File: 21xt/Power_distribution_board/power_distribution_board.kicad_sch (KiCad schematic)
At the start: 38 parts, among them IC1 LM74700QDBVRQ1, IC2 LM74700QDBVRQ1, IC3 LTC2959IDDB#TRMPBF, IC4 INA180A1IDBVR, IC5 TLV76150DCYR, J1 Conn_01x02, J2 Conn_01x02, J3 Conn_01x02, J4 Conn_01x02, J5 Conn_01x02, Q1 NVMFWS2D1N08XT1G, Q2 NVMFWS2D1N08XT1G, Q3 NVMFWS2D1N08XT1G, U1 esp32 c6 xiao, U2 LMV331

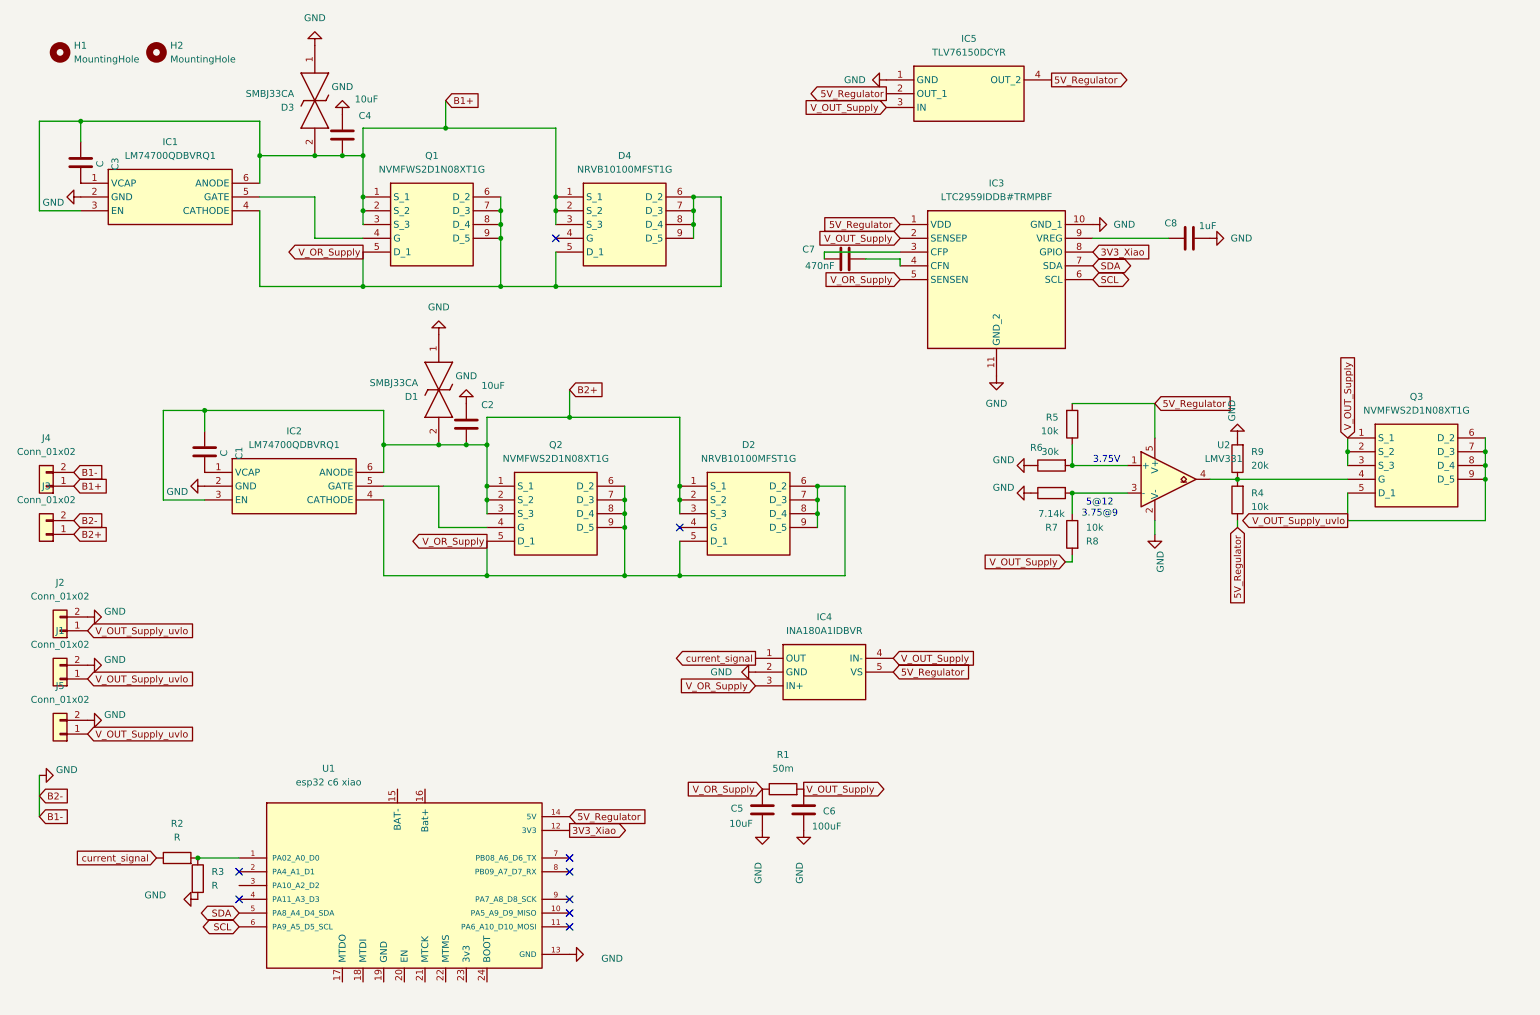
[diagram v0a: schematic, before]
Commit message: done i hope
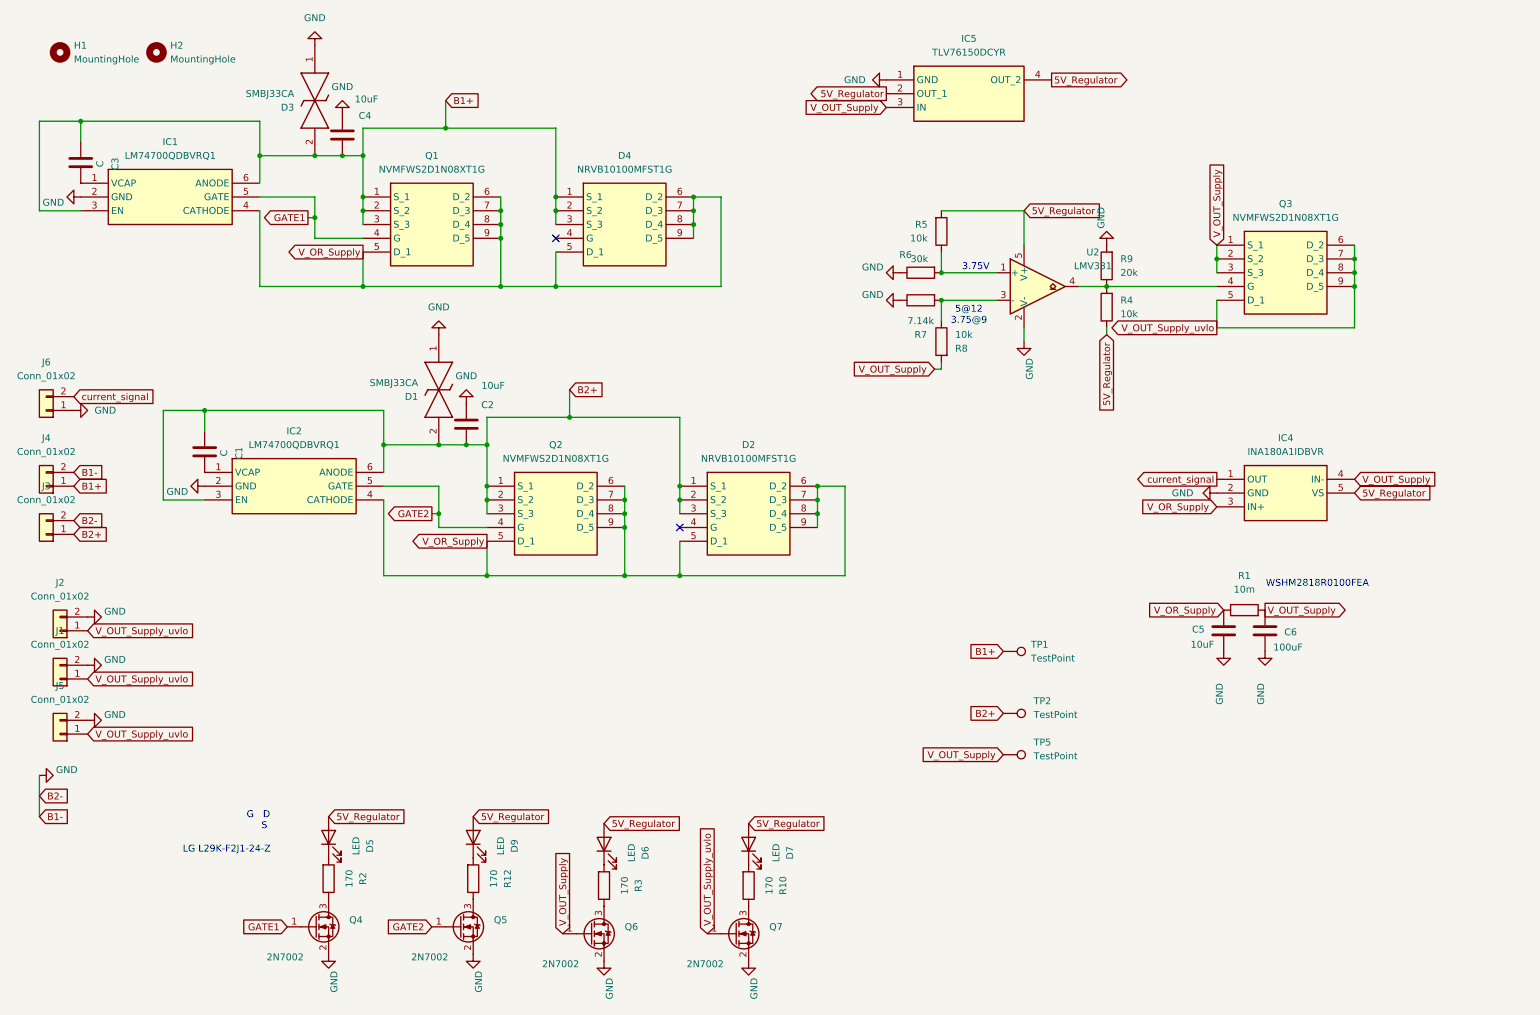
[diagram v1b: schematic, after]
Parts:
- removed C7: 470nF, Capacitor_SMD:C_0402_1005Metric, symbol Device:C
- removed C8: 1uF, Capacitor_SMD:C_0402_1005Metric, symbol Device:C
- removed IC3: LTC2959IDDB#TRMPBF, 21xt_footprints:LTC2959IDDB#TRMPBF, symbol 21xt_symbols:LTC2959IDDB#TRMPBF
- removed U1: esp32 c6 xiao, 21xt_footprints:esp32 c6 smt, symbol 21xt_symbols:102010388
- added D5, D6, D7, D9: LED, LED_SMD:LED_0603_1608Metric, symbol Device:LED
- added J6: Conn_01x02, Connector_JST:JST_EH_S2B-EH_1x02_P2.50mm_Horizontal, symbol Connector_Generic:Conn_01x02
- added Q4, Q5, Q6, Q7: 2N7002, Package_TO_SOT_SMD:SOT-23, symbol Transistor_FET:2N7002
- added R10, R12: 170, Resistor_SMD:R_0402_1005Metric, symbol Device:R
- added TP1, TP2, TP5: TestPoint, TestPoint:TestPoint_Pad_1.0x1.0mm, symbol Connector:TestPoint
- R1: value 50m -> 10m
- R2, R3: value R -> 170
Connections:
- net 5V_Regulator: now also D5.2 (A), D6.2 (A), D7.2 (A), D9.2 (A)
- net B1+: now also TP1.1
- net B2+: now also TP2.1
- net GND: now also J6.1 (Pin_1), Q4.2 (S), Q5.2 (S), Q6.2 (S), Q7.2 (S); no longer R3.2
- net V_OUT_Supply: now also Q6.1 (G), TP5.1
- net V_OUT_Supply_uvlo: now also Q7.1 (G)
- net current_signal: now also J6.2 (Pin_2); no longer R2.1
- net GATE2: now reaches IC2.5 (GATE), Q2.4 (G)
- net GATE2: now also Q5.1 (G)
- net at R3.1: now also Q6.3 (D); no longer R2.2
- net GATE1: now reaches IC1.5 (GATE), Q1.4 (G)
- net GATE1: now also Q4.1 (G)
- new net: Q7.3 (D), R10.1
- new net: D7.1 (K), R10.2
- new net: D5.1 (K), R2.2
- new net: Q5.3 (D), R12.1
- new net: D6.1 (K), R3.2
- new net: Q4.3 (D), R2.1
- new net: D9.1 (K), R12.2
- no-connect marks 9 -> 2
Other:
- note added: "G D S"
- note added: "LG L29K-F2J1-24-Z"
- note added: "WSHM2818R0100FEA"
- moved on the sheet: C5, C6, IC4, Q3, R1, R4, R5, R6, R7, R8, R9, U2

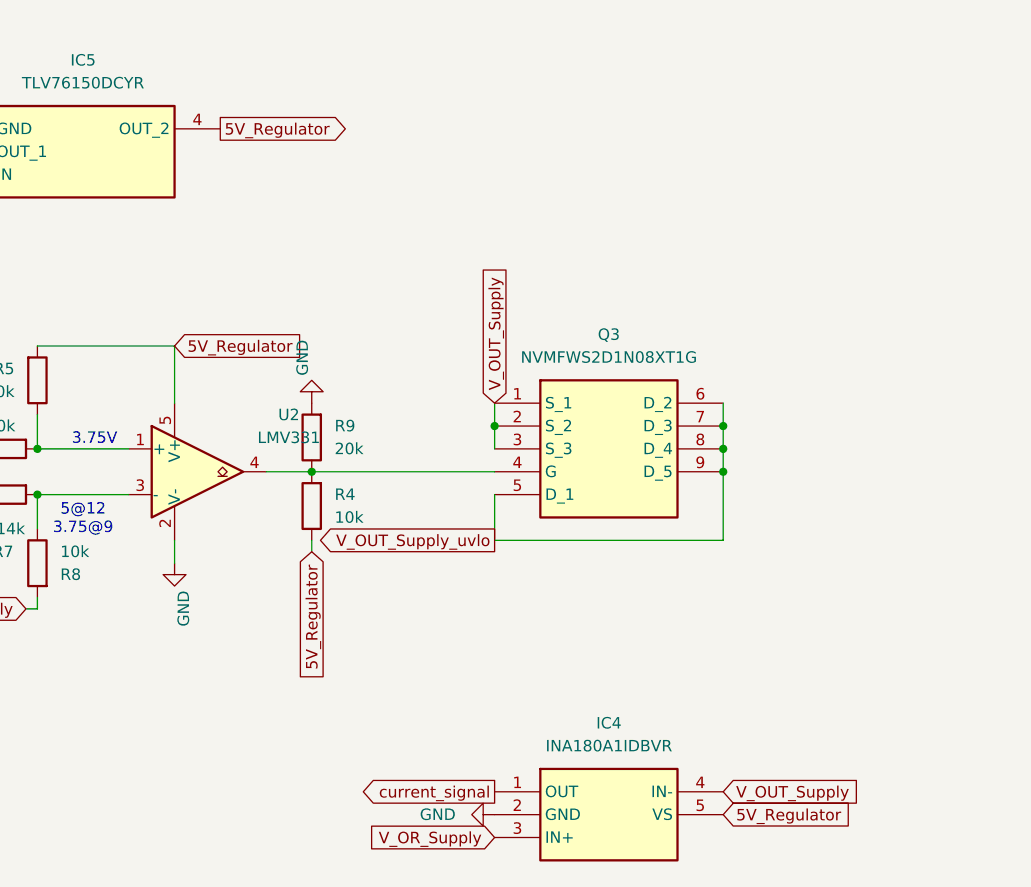
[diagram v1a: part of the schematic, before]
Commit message: adf
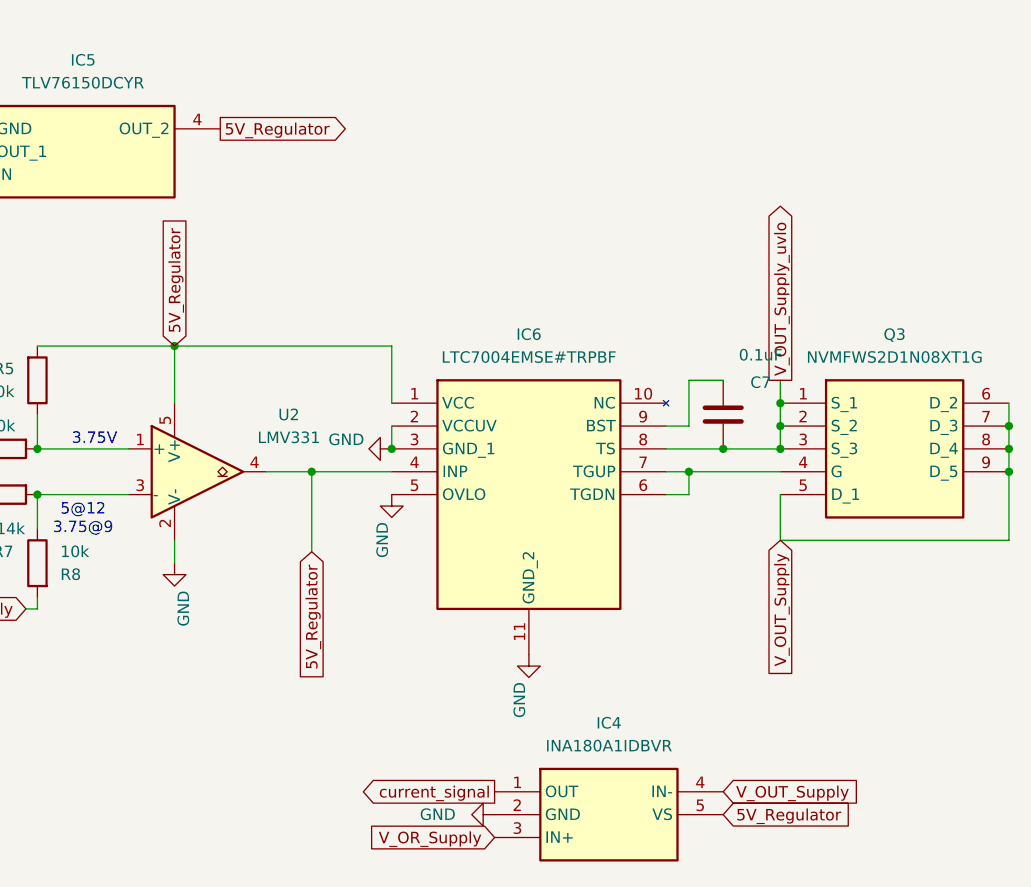
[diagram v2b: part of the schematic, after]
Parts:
- removed R4: 10k, Resistor_SMD:R_0402_1005Metric, symbol Device:R
- removed R9: 20k, Resistor_SMD:R_0402_1005Metric, symbol Device:R
- added C7: 0.1uF, Capacitor_SMD:C_0402_1005Metric, symbol Device:C
- added IC6: LTC7004EMSE#TRPBF, deans_fp:SOP50P490X110-11N, symbol ihatekicad:LTC7004EMSE#TRPBF
- J1, J2, J5: footprint 21xt_footprints:Deans Connector Female -> deans_fp:Deans Connector Female
- J3, J4: footprint 21xt_footprints:Deans Connector Male -> deans_fp:Deans Connector Male
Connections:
- net 5V_Regulator: now also U2.4, IC6.1 (VCC), IC6.4 (INP)
- net GND: now also IC6.11 (GND_2), IC6.2 (VCCUV), IC6.3 (GND_1), IC6.5 (OVLO)
- net V_OUT_Supply: now also Q3.5 (D_1), Q3.6 (D_2), Q3.7 (D_3), Q3.8 (D_4), Q3.9 (D_5); no longer Q3.1 (S_1), Q3.2 (S_2), Q3.3 (S_3)
- net V_OUT_Supply_uvlo: now also Q3.1 (S_1), Q3.2 (S_2), Q3.3 (S_3), C7.2, IC6.8 (TS); no longer Q3.5 (D_1), Q3.6 (D_2), Q3.7 (D_3), Q3.8 (D_4), Q3.9 (D_5)
- net at Q3.4 (G): now also IC6.6 (TGDN), IC6.7 (TGUP); no longer U2.4
- new net: C7.1, IC6.9 (BST)
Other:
- moved on the sheet: Q3
